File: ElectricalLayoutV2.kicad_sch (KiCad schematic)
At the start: 19 parts, among them U1 DS18B20, U2 DS18B20, U3 DS18B20, U4 DS18B20

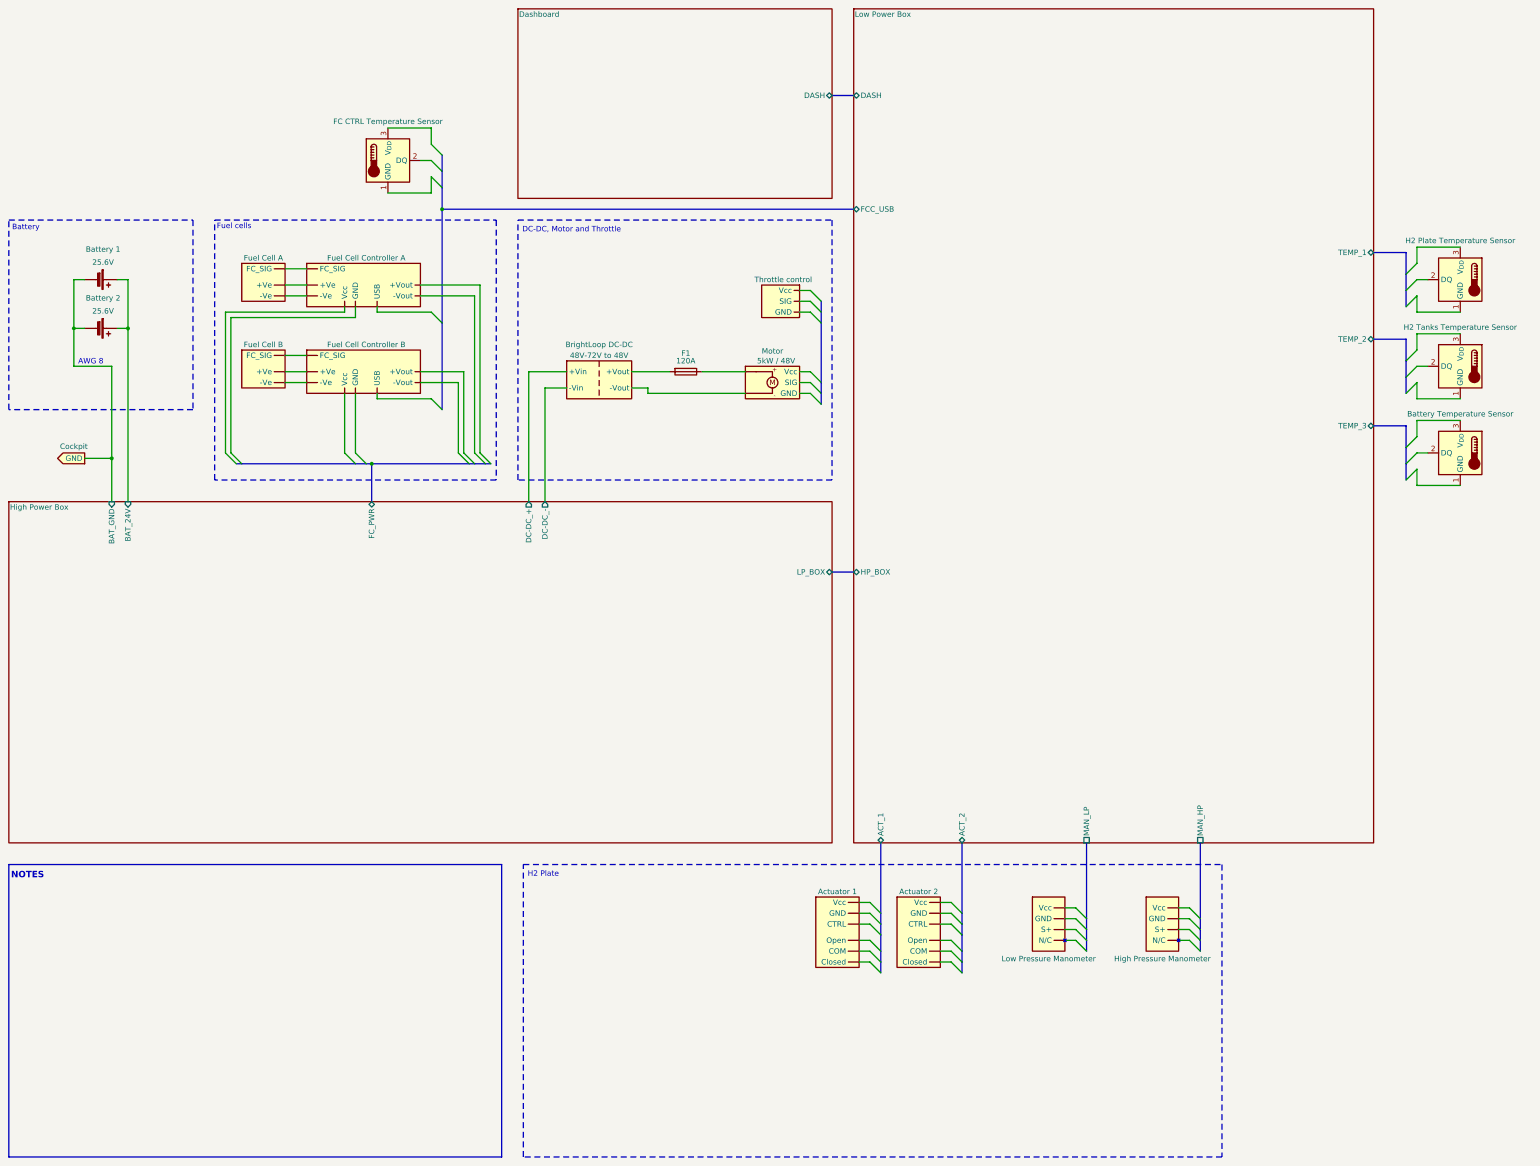
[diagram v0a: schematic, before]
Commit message: Finalize layout
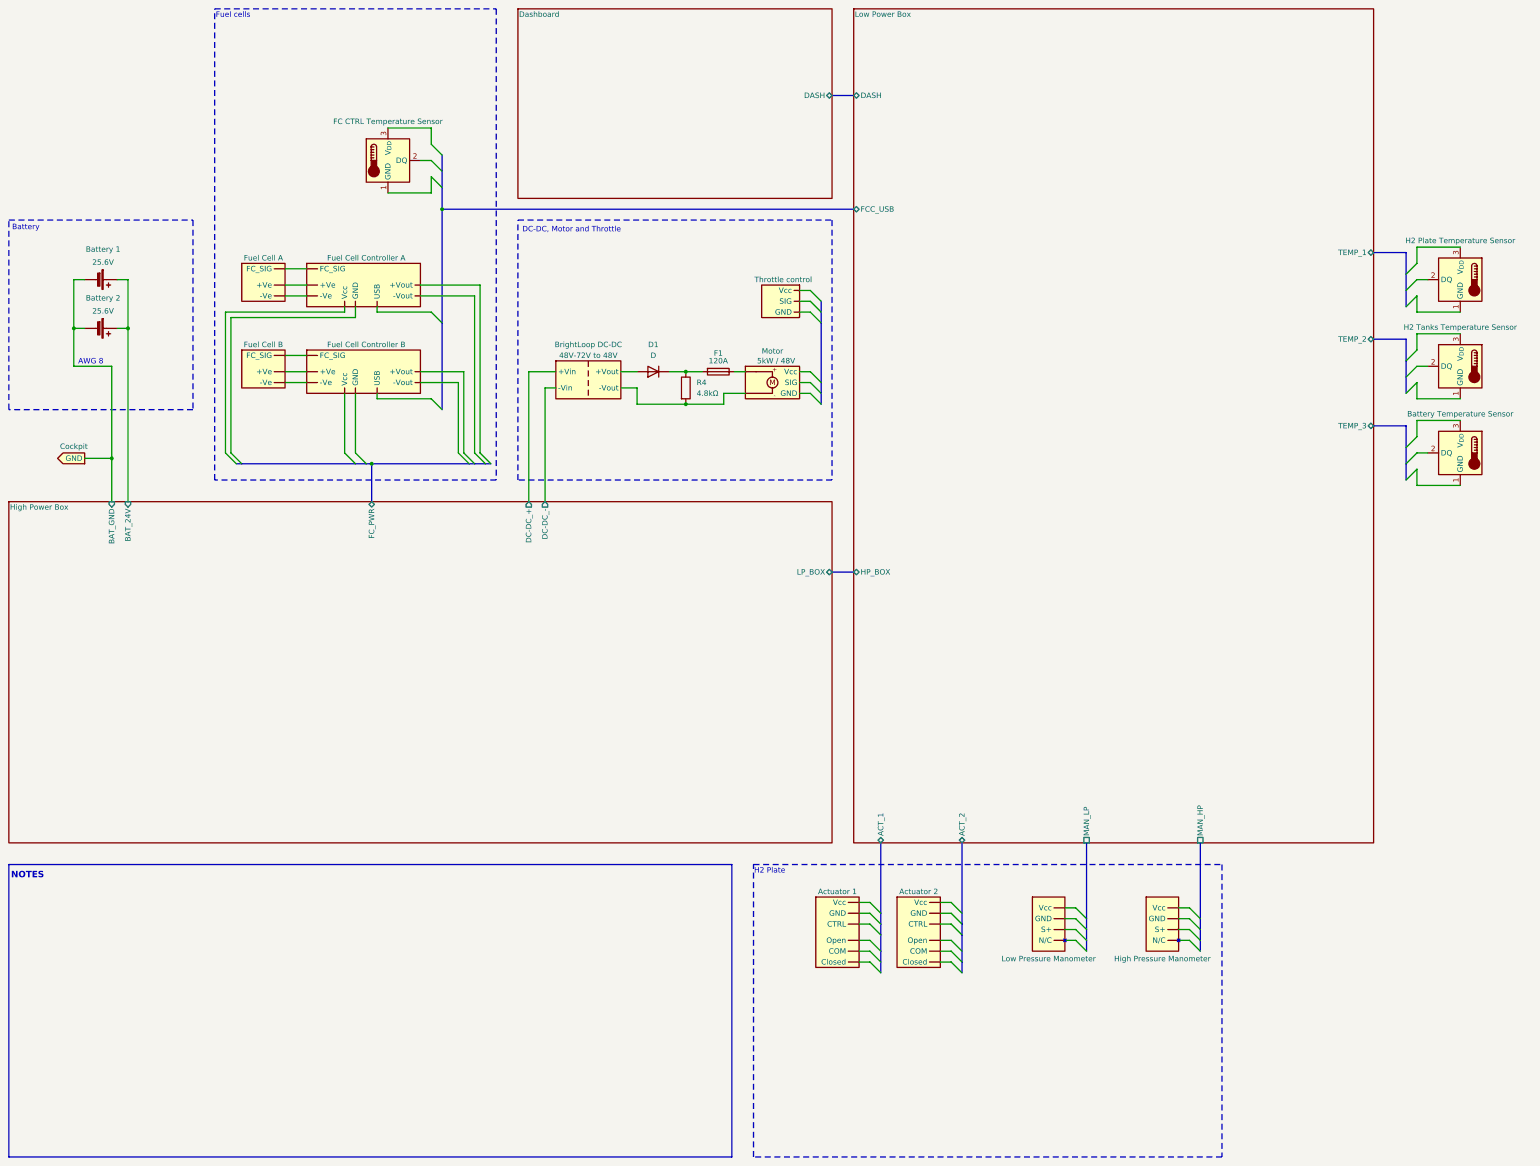
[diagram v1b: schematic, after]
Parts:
- added D1: D, symbol Device:D
- added R4: 4.8kΩ, symbol Device:R
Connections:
- net at F1.2: now also D1.1 (K), R4.1; no longer DCC1. (-Vout)
- net at FCC1. (Vcc): no longer FC1. (FC_SIG)
- net at PROP1. (Vcc): now also DCC1. (-Vout), R4.2
- net at FCC2. (Vcc): now also FC2. (FC_SIG)
- new net: FC1. (FC_SIG), FCC1. (Vcc) (x2)
- new net: FC2. (FC_SIG), FCC2. (Vcc) (x2)
- new net: D1.2 (A), DCC1. (-Vout)
- now unconnected: FCC1. (Vcc)
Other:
- moved on the sheet: F1
